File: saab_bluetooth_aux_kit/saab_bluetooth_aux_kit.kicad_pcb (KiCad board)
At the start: 2 copper layers, 3 parts, among them U1 CC3-0505SF-E, U2 ESP32-WROOM-DEVKIT, U4 UDA1334A_BREAKOUT

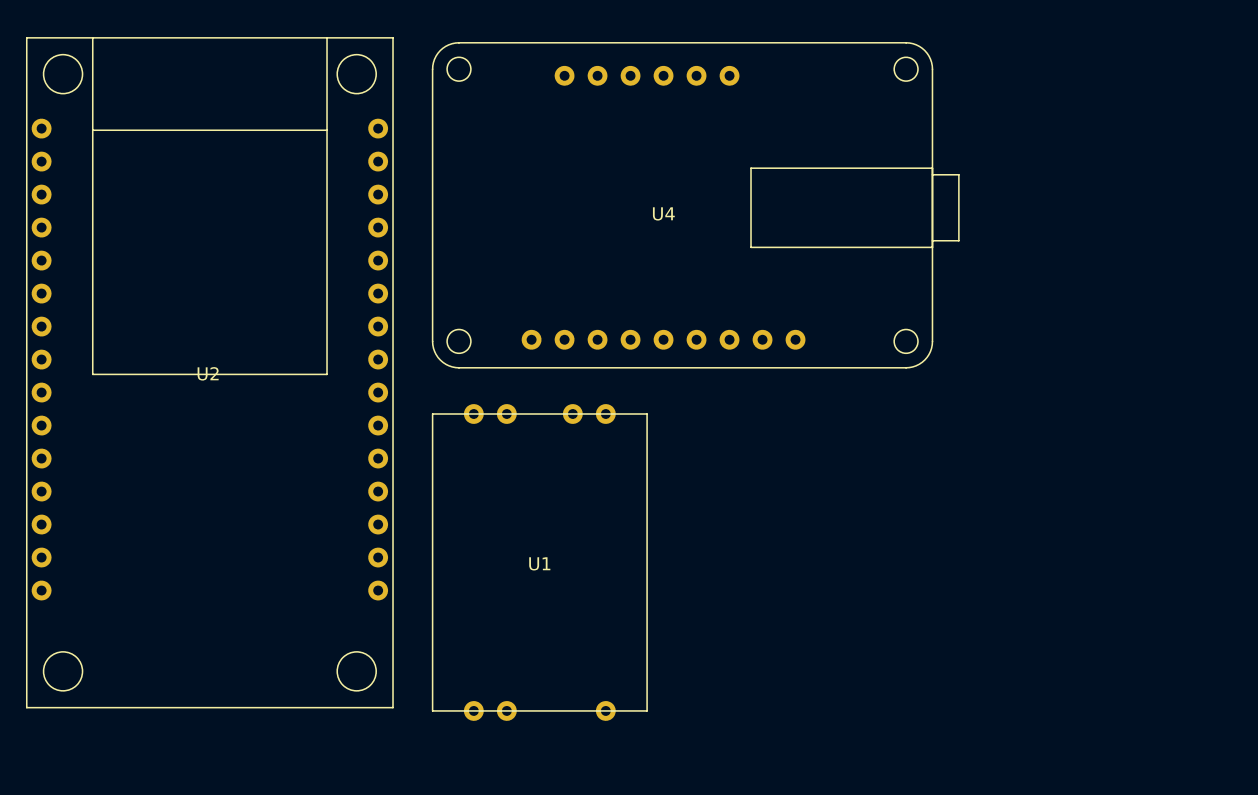
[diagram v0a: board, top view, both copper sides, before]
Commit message: Made simple PCB
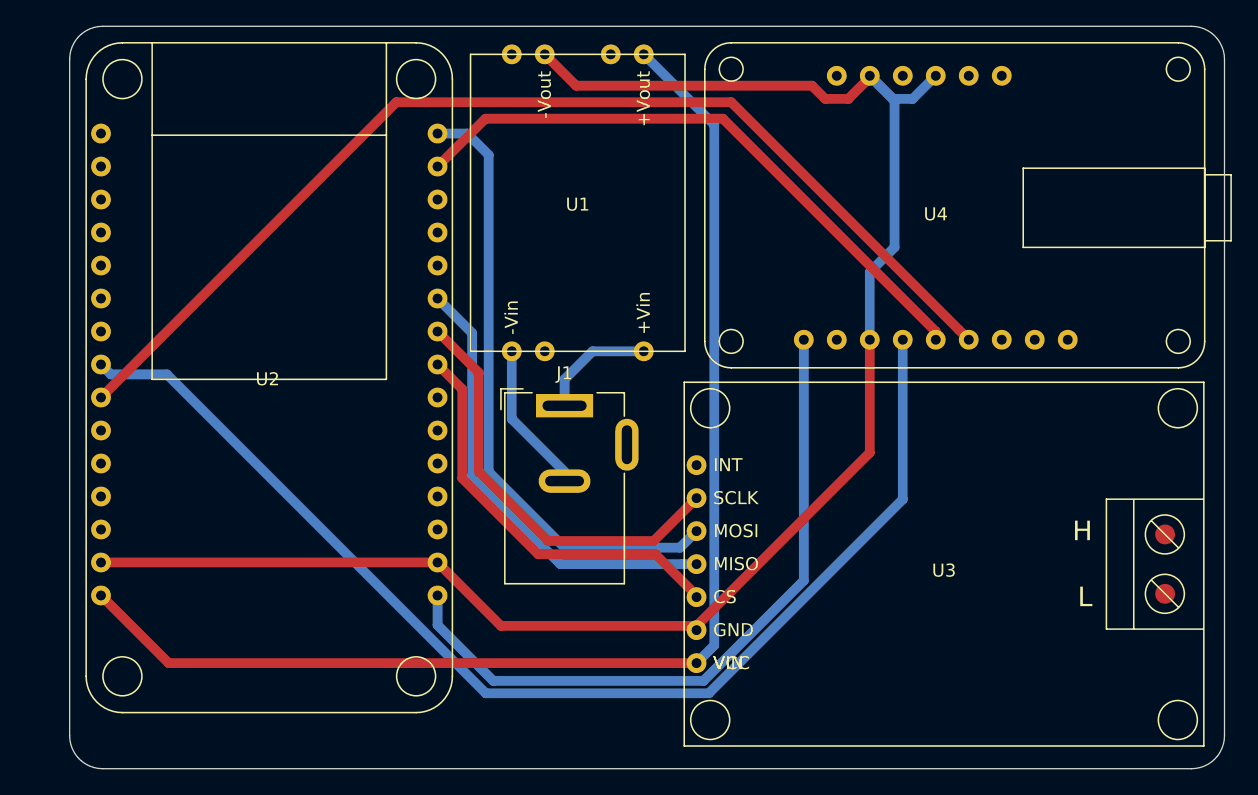
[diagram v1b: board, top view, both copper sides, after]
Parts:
- added J1: Barrel_Jack, Connector_BarrelJack:BarrelJack_Wuerth_6941xx301002, F.Cu at (133.3, 104.1)
- added U3: MCP2515_MODULE, custom_footprints:MCP2515_Module, F.Cu at (162.6, 116.3)
- U2: value ESP32-WROOM-DEVKIT -> ESP32-WROOM-DEVKIT-custom_symbols
- moved U1 27.8 mm to (134.4, 89.2)
- moved U4 21.0 mm to (161.9, 88.9)
- moved U2 4.59 mm to (110.5, 101.6)
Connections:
- U1 pad 1: (no net) -> Net-(J1-Pad1)
- U1 pad 3: (no net) -> Net-(J1-Pad2)
- U1 pad 5: (no net) -> GND
- U1 pad 7: (no net) -> 5VDC
- U2 pad 3V3: (no net) -> 3VDC
- U2 pad GND: (no net) -> GND
- U2 pad GPIO18: (no net) -> SPI_SCLK
- U2 pad GPIO19: (no net) -> SPI_MISO
- U2 pad GPIO22: (no net) -> I2S_DIN
- U2 pad GPIO23: (no net) -> SPI_MOSI
- U2 pad GPIO25: (no net) -> I2S_WSEL
- U2 pad GPIO26: (no net) -> I2S_BCLK
- U2 pad GPIO5: (no net) -> SPI_CS
- U2 pad VIN: (no net) -> 5VDC
- U4 pad BCLK: (no net) -> I2S_BCLK
- U4 pad DIN: (no net) -> I2S_DIN
- U4 pad GND: (no net) -> GND
- U4 pad SF0: (no net) -> GND
- U4 pad SF1: (no net) -> GND
- U4 pad VIN: (no net) -> 3VDC
- U4 pad WSEL: (no net) -> I2S_WSEL
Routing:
- net GND: track 0.00 -> 131.4 mm
- net 5VDC: track 0.00 -> 97.7 mm
- net I2S_WSEL: track 0.00 -> 90.7 mm
- net I2S_BCLK: track 0.00 -> 83.8 mm
- net 3VDC: track 0.00 -> 54.0 mm
- net SPI_MOSI: track 0.00 -> 48.0 mm
- net I2S_DIN: track 0.00 -> 47.3 mm
- net SPI_MISO: track 0.00 -> 34.8 mm
- net SPI_SCLK: track 0.00 -> 32.5 mm
- net SPI_CS: track 0.00 -> 31.4 mm
- net Net-(J1-Pad2): track 0.00 -> 11.7 mm
- net Net-(J1-Pad1): track 0.00 -> 9.02 mm
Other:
- board outline added: 88.9 x 57.2 mm
